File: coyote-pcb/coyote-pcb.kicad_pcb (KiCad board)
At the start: 2 copper layers, 106 x 47 mm, 17 parts, among them U1 Basalt

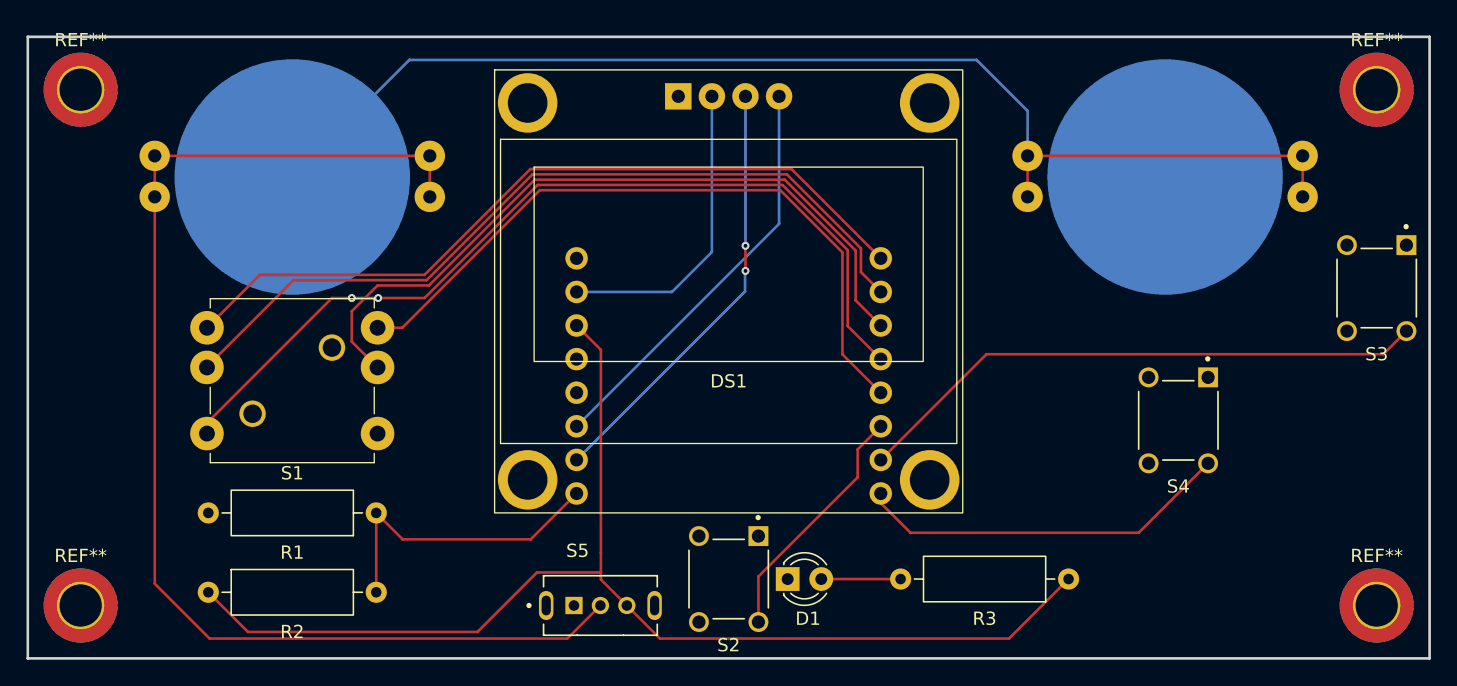
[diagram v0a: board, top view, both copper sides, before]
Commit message: Update with new Basalt design
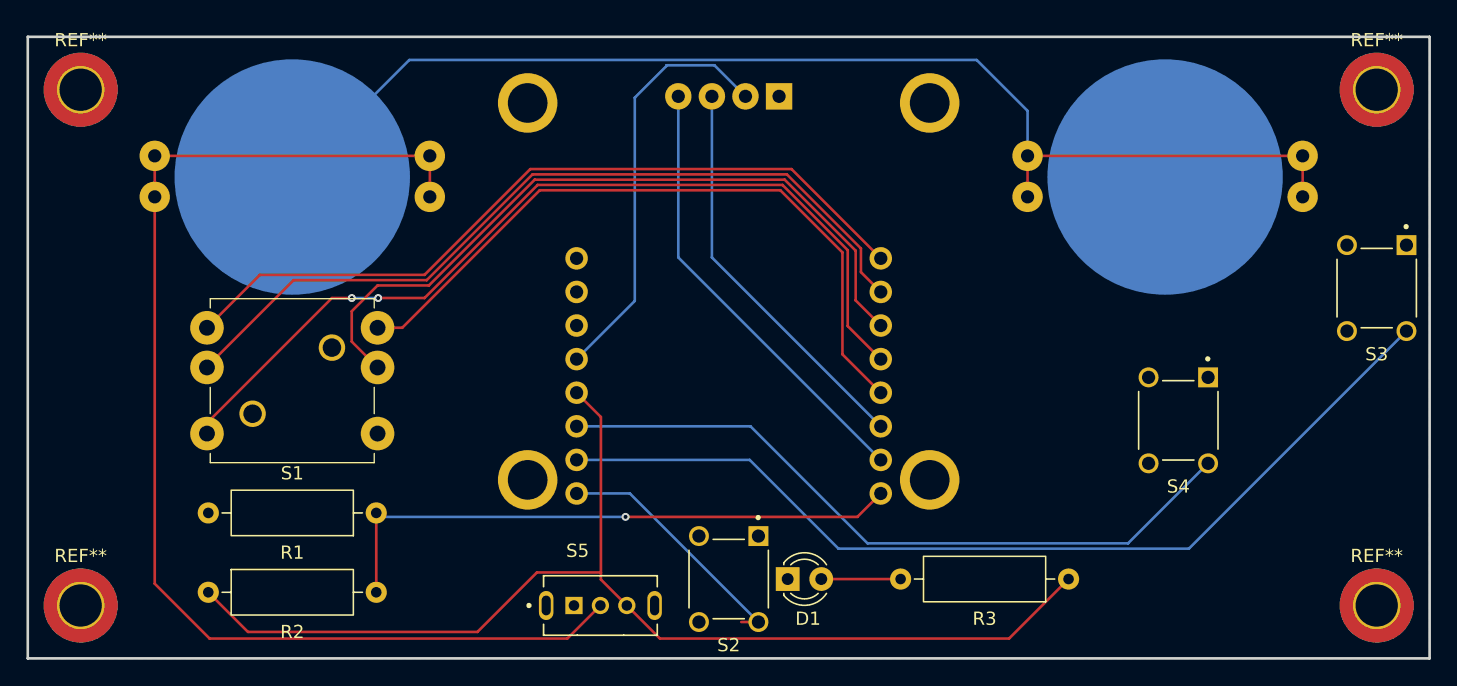
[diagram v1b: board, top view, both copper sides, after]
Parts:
- DS1: moved to B.Cu
- turned DS1 to 180 degrees
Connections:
- U1 pad 10: Net-(DS1-SCL) -> Net-(S3-Pad2)
- U1 pad 11: Net-(DS1-SDA) -> Net-(S4-Pad2)
- U1 pad 12: unconnected-(U1-Pad12) -> +5V
- U1 pad 13: unconnected-(U1-Pad13) -> +3.3V
- U1 pad 14: +5V -> GND
- U1 pad 15: +3.3V -> (no net)
- U1 pad 16: GND -> (no net)
- U1 pad 6: Net-(S2-Pad2) -> Net-(DS1-SCL)
- U1 pad 7: Net-(S3-Pad2) -> Net-(DS1-SDA)
- U1 pad 8: Net-(S4-Pad2) -> Net-(R1-Pad1)
- U1 pad 9: Net-(R1-Pad1) -> Net-(S2-Pad2)
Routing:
- net Net-(S3-Pad2): track 43.8 -> 72.3 mm
- net Net-(S4-Pad2): track 28.6 -> 53.9 mm
- net Net-(R1-Pad1): track 23.4 -> 45.7 mm, vias 0 -> 1
- net +3.3V: track 23.3 -> 32.0 mm
- net +5V: track 92.2 -> 87.1 mm
- net Net-(DS1-SCL): track 32.8 -> 30.2 mm, vias 2 -> 0
- net Net-(DS1-SDA): track 31.3 -> 33.8 mm
